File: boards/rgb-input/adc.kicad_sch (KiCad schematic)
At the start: 9 parts, among them U13 MCP1502, U2 MCP3208, U4 MCP3221A0T

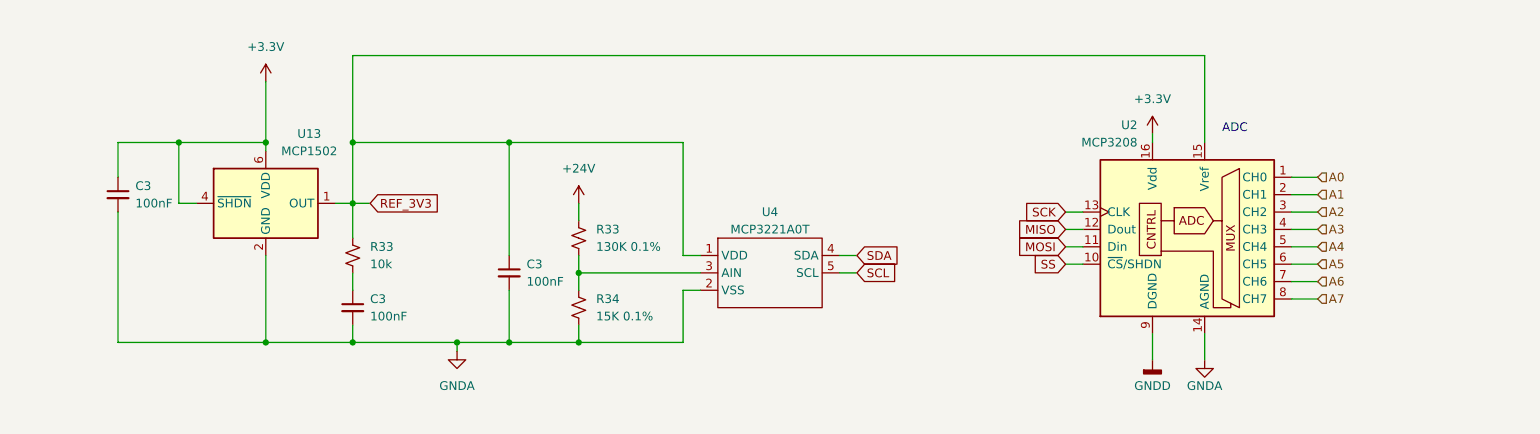
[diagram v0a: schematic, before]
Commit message: some adc changes and then rerouting
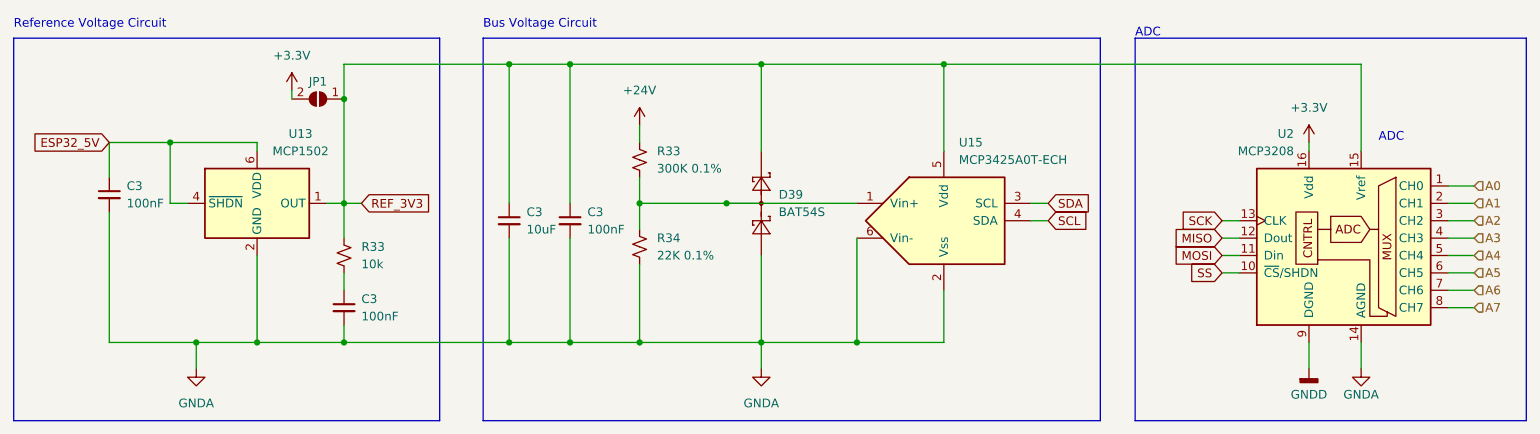
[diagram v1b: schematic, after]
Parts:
- removed U4: MCP3221A0T, Package_TO_SOT_SMD:SOT-23-5, symbol gnarboard:MCP3X21
- added C3: 10uF, Capacitor_SMD:C_0805_2012Metric_Pad1.18x1.45mm_HandSolder, symbol Device:C_Small
- added D39: BAT54S, Package_TO_SOT_SMD:SOT-23, symbol Diode:BAT54S
- added JP1: SolderJumper_2_Open, Jumper:SolderJumper-2_P1.3mm_Open_RoundedPad1.0x1.5mm, symbol Jumper:SolderJumper_2_Open
- added U15: MCP3425A0T-ECH, Package_TO_SOT_SMD:SOT-23-6, symbol Analog_ADC:MCP3425A0T-ECH
- R33: value 130K 0.1% -> 300K 0.1%
- R34: value 15K 0.1% -> 22K 0.1%
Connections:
- net +3.3V: now also JP1.2 (B); no longer C3.1, U13.4 (~{SHDN}), U13.6 (VDD)
- net GNDA: now also C3.2, D39.1 (A), U15.2 (Vss), U15.6 (Vin-)
- net REF_3V3: now also C3.1, D39.2 (K), JP1.1 (A), U15.5 (Vdd)
- net SCL: now also U15.4 (SDA)
- net SDA: now also U15.3 (SCL)
- net at R33.1, R34.2: now also D39.3 (COM), U15.1 (Vin+)
- new net ESP32_5V: C3.1, U13.4 (~{SHDN}), U13.6 (VDD)
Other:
- note added: "Bus Voltage Circuit"
- note added: "Reference Voltage Circuit"
- moved on the sheet: C3, R33, R34, U13, U2

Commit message: too much routing
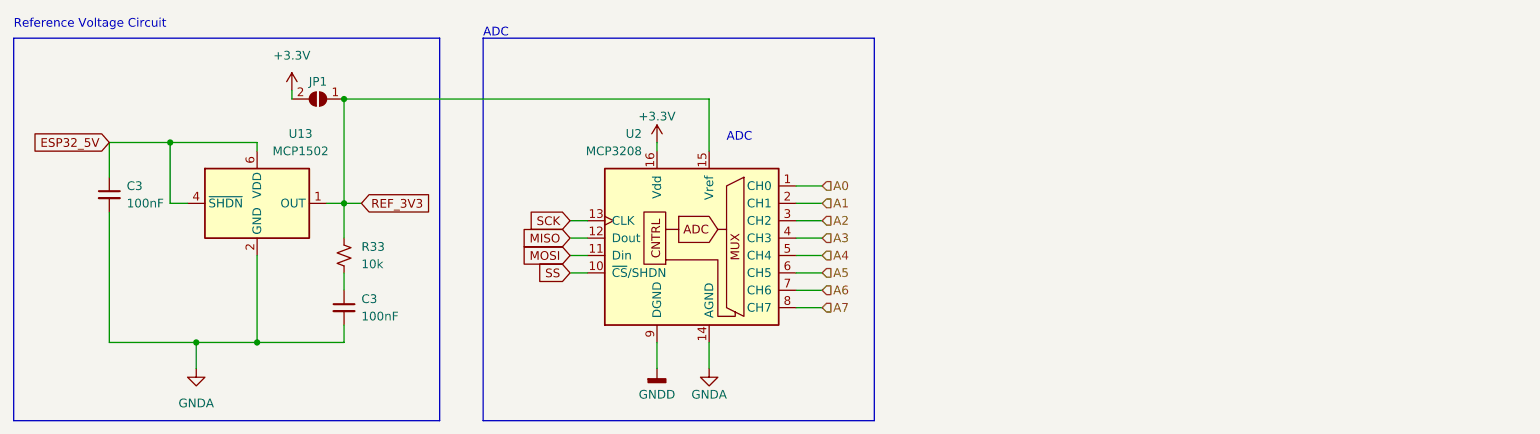
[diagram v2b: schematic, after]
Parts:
- removed C3: 10uF, Capacitor_SMD:C_0805_2012Metric_Pad1.18x1.45mm_HandSolder, symbol Device:C_Small
- removed C3: 100nF, Capacitor_SMD:C_0805_2012Metric_Pad1.18x1.45mm_HandSolder, symbol Device:C_Small
- removed D39: BAT54S, Package_TO_SOT_SMD:SOT-23, symbol Diode:BAT54S
- removed R33: 300K 0.1%, Resistor_SMD:R_0805_2012Metric_Pad1.20x1.40mm_HandSolder, symbol Device:R_Small_US
- removed R34: 22K 0.1%, Resistor_SMD:R_0805_2012Metric_Pad1.20x1.40mm_HandSolder, symbol Device:R_Small_US
- removed U15: MCP3425A0T-ECH, Package_TO_SOT_SMD:SOT-23-6, symbol Analog_ADC:MCP3425A0T-ECH
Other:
- note removed: "Bus Voltage Circuit"
- moved on the sheet: U2
